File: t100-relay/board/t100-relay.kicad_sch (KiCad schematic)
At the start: 14 parts, among them J1 T100-IN, J2 T100-OUT, J3 Conn_01x02_Female, J4 Conn_01x02_Female, K1 RELAY_2, Q1 BC817, U1 ATSAMD09C13A-SS, X1 SWD

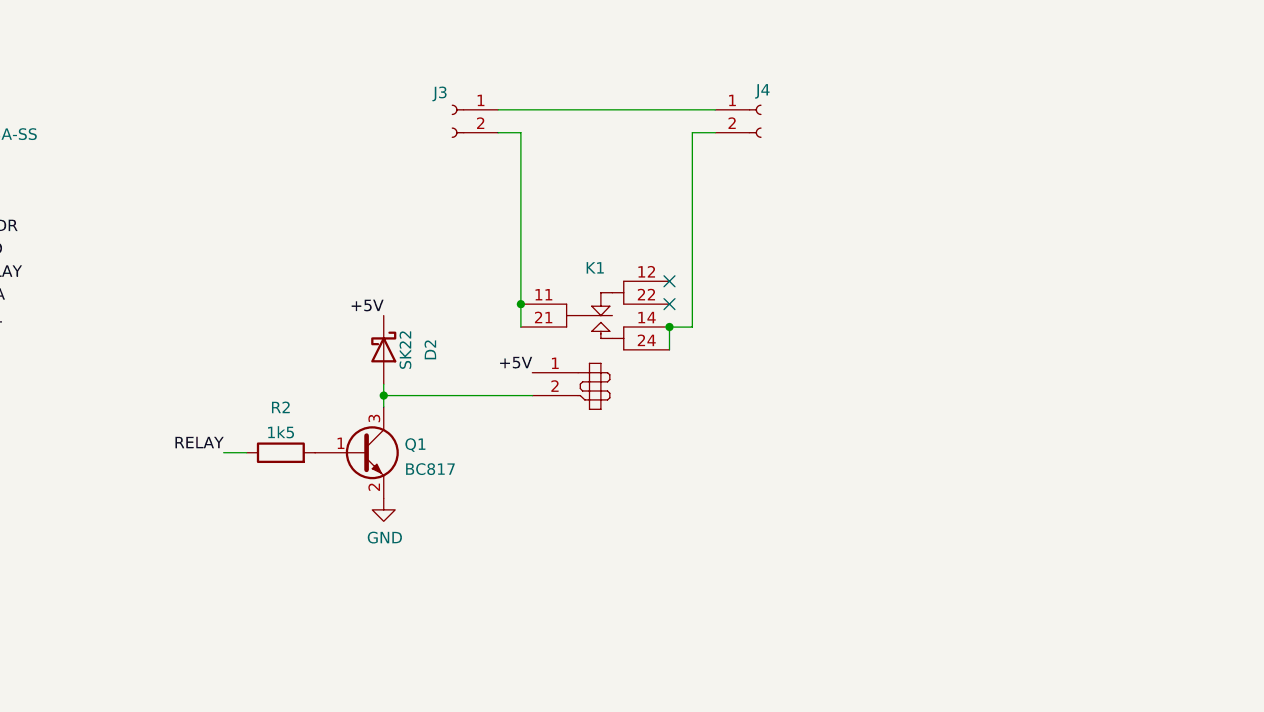
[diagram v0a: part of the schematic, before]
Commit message: WIP
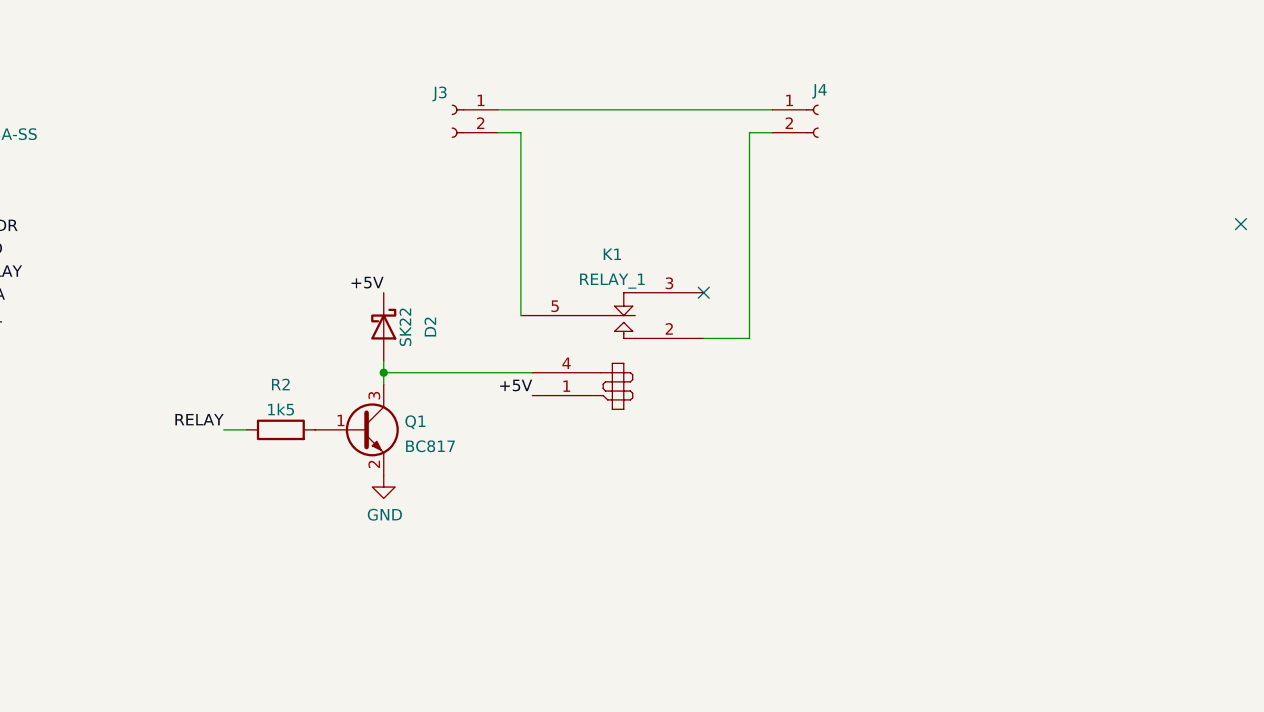
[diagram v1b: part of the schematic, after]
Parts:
- removed K1: RELAY_2, Drake:RT314_Relay, symbol Drake:RELAY_2
- added K1: RELAY_1, Drake:SRD_C_Relay, symbol Drake:RELAY_1
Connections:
- net +5V: now also K1.1 (C2)
- net at D2.2 (A), Q1.3 (C): now also K1.4 (C1)
- net at J4.2 (Pin_2): now also K1.2 (B)
- net at J3.2 (Pin_2): now also K1.5 (A)
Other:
- moved on the sheet: D2, J4, Q1, R2
